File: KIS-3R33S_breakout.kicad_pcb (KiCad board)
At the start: 2 copper layers, 5 parts, among them P1 Screw terminal, P2 Screw terminal, U1 KIS-3R33S_modif

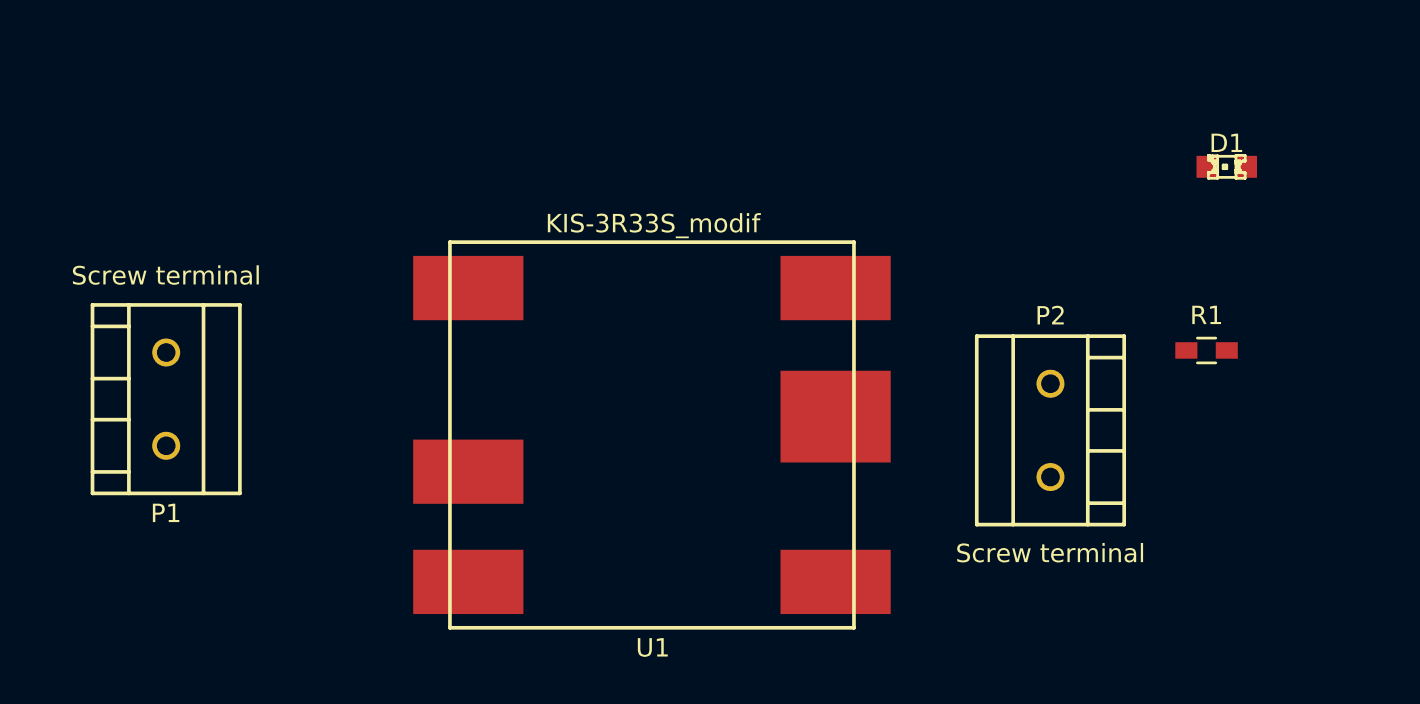
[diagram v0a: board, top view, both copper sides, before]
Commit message: Throwing parts around.
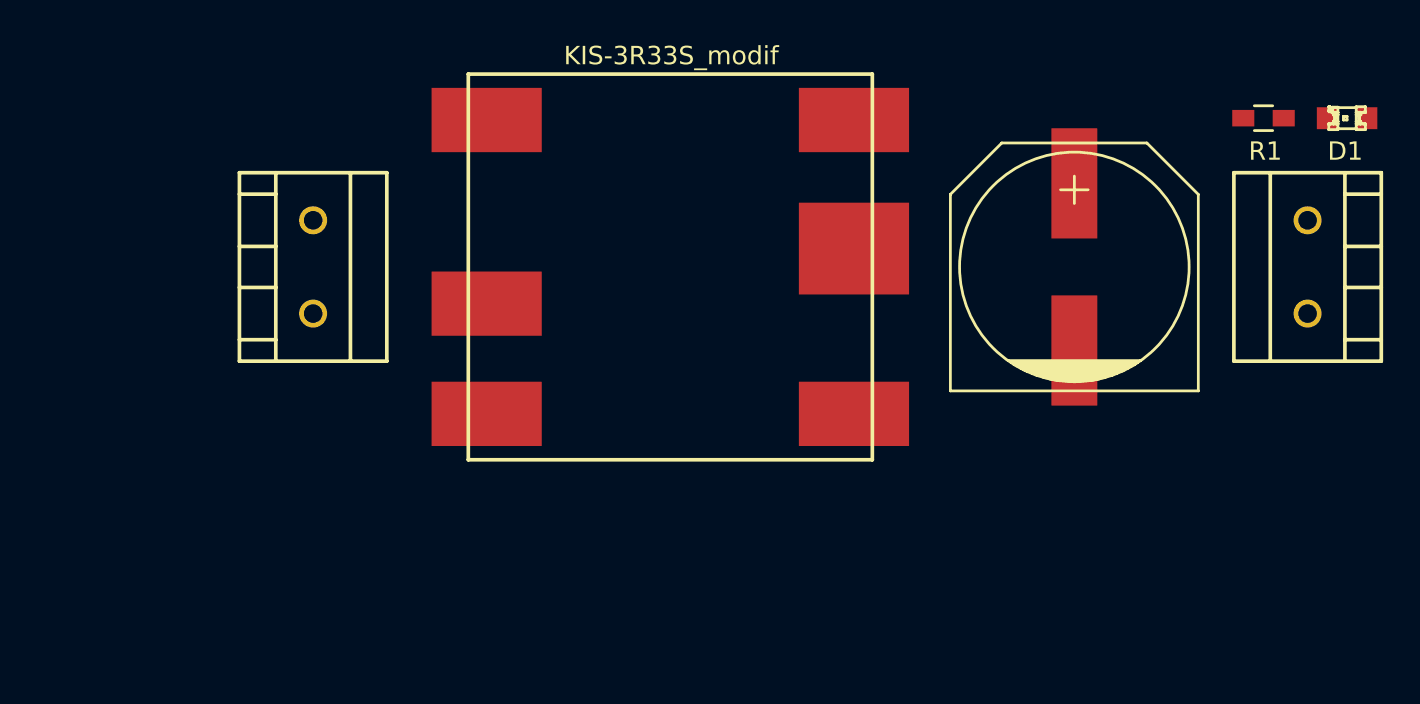
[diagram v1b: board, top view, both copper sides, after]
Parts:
- added C1: 1mF, 25V, Capacitors_SMD:c_elec_SMD_12.5x13.5, F.Cu at (172.0, 100.0)
- moved P2 16.6 mm to (184.7, 100.0)
- moved R1 13.0 mm to (182.3, 91.9)
- moved P1 10.8 mm to (130.6, 100.0)
- moved U1 9.20 mm to (150.0, 100.0)
- moved D1 7.07 mm to (186.8, 91.9)
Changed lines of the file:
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@@
 (kicad_pcb (version 4) (host pcbnew "(2015-05-01 BZR 5636)-product")
   (general
-    (links 8)
-    (no_connects 8)
-    (area 116.607142 92.155 182.14846 121.75)
+    (links 10)
+    (no_connects 10)
+    (area 124.607142 87.3 190.642858 112.6)
     (thickness 1.6)
     (drawings 0)
     (tracks 0)
     (zones 0)
-    (modules 5)
+    (modules 6)
     (nets 5)
   )
@@
   )
   (module DC-DC-modules:KIS-3R33S (layer F.Cu)
-    (at 149 109.15)
+    (at 150 100)
     (descr ./Docs/KIS-3R33S.pdf)
     (tags "DC-DC, buck, KIS-3R33S")
-    (fp_text reference U1 (at 0.05 11.6) (layer F.SilkS)
+    (fp_text reference U1 (at 0.05 11.6) (layer F.SilkS) hide
       (effects (font (size 1 1) (thickness 0.2)))
     )
@@
   )
   (module LEDs:LED-0805 (layer F.Cu)
-    (at 180.3 94.55)
+    (at 186.85 91.9)
     (descr "LED 0805 smd package")
     (tags "LED 0805 SMD")
     (attr smd)
-    (fp_text reference D1 (at 0 -1.27) (layer F.SilkS)
+    (fp_text reference D1 (at -0.1 1.8) (layer F.SilkS)
       (effects (font (size 1 1) (thickness 0.15)))
     )
@@
   )
   (module my_parts:MADW__SCREW_TERMINAL_2pin (layer F.Cu)
-    (at 122.55 107.2 180)
-    (fp_text reference P1 (at 0.01 -6.23 180) (layer F.SilkS)
-      (effects (font (size 1 1) (thickness 0.2)))
-    )
-    (fp_text value "Screw terminal" (at 0 6.71 180) (layer F.SilkS)
+    (at 130.55 100 180)
+    (fp_text reference P1 (at 0.01 -6.23 180) (layer F.SilkS) hide
+      (effects (font (size 1 1) (thickness 0.2)))
+    )
+    (fp_text value "Screw terminal" (at 0 6.71 180) (layer F.SilkS) hide
       (effects (font (size 1 1) (thickness 0.2)))
     )
@@
   )
   (module my_parts:MADW__SCREW_TERMINAL_2pin (layer F.Cu)
-    (at 170.7 108.9)
-    (fp_text reference P2 (at 0.01 -6.23) (layer F.SilkS)
-      (effects (font (size 1 1) (thickness 0.2)))
-    )
-    (fp_text value "Screw terminal" (at 0 6.71) (layer F.SilkS)
+    (at 184.7 100)
+    (fp_text reference P2 (at 0.01 -6.23) (layer F.SilkS) hide
+      (effects (font (size 1 1) (thickness 0.2)))
+    )
+    (fp_text value "Screw terminal" (at 0 6.71) (layer F.SilkS) hide
       (effects (font (size 1 1) (thickness 0.2)))
     )
@@
   )
   (module Resistors_SMD:R_0603_HandSoldering (layer F.Cu)
-    (at 179.2 104.55)
+    (at 182.3 91.9)
     (descr "Resistor SMD 0603, hand soldering")
     (tags "resistor 0603")
     (attr smd)
-    (fp_text reference R1 (at 0 -1.9) (layer F.SilkS)
+    (fp_text reference R1 (at 0.1 1.8) (layer F.SilkS)
       (effects (font (size 1 1) (thickness 0.15)))
     )
@@
     )
   )
+  (module Capacitors_SMD:c_elec_SMD_12.5x13.5 (layer F.Cu)
+    (at 172 100 90)
+    (descr "SMT capacitor, aluminium electrolytic, 12.5x13.5")
+    (fp_text reference C1 (at 8.6 -0.05 180) (layer F.SilkS) hide
+      (effects (font (size 1 1) (thickness 0.15)))
+    )
+    (fp_text value "1mF, 25V" (at 0 8 90) (layer F.Fab) hide
+      (effects (font (size 1 1) (thickness 0.15)))
+    )
+    (fp_line (start 3.95 -6.75) (end 6.75 -3.95) (layer F.SilkS) (width 0.15))
+    (fp_line (start 6.75 3.95) (end 3.95 6.75) (layer F.SilkS) (width 0.15))
+    (fp_line (start -6.15 1.1) (end -6.15 -1.1) (layer F.SilkS) (width 0.15))
+    (fp_line (start -6.1 1.35) (end -6.1 -1.35) (layer F.SilkS) (width 0.15))
+    (fp_line (start -6 -1.7) (end -6 1.7) (layer F.SilkS) (width 0.15))
+    (fp_line (start -5.9 2.05) (end -5.9 -2.05) (layer F.SilkS) (width 0.15))
+    (fp_line (start -5.8 -2.3) (end -5.8 2.3) (layer F.SilkS) (width 0.15))
+    (fp_line (start -5.7 2.55) (end -5.7 -2.55) (layer F.SilkS) (width 0.15))
+    (fp_line (start -5.6 2.75) (end -5.6 -2.75) (layer F.SilkS) (width 0.15))
+    (fp_line (start -5.5 -2.95) (end -5.5 2.95) (layer F.SilkS) (width 0.15))
+    (fp_line (start -5.4 3.1) (end -5.4 -3.1) (layer F.SilkS) (width 0.15))
+    (fp_line (start -5.3 -3.3) (end -5.3 3.3) (layer F.SilkS) (width 0.15))
+    (fp_line (start -5.2 -3.45) (end -5.2 3.45) (layer F.SilkS) (width 0.15))
+    (fp_line (start -5.1 -3.6) (end -5.1 3.6) (layer F.SilkS) (width 0.15))
+    (fp_line (start -2.2 -0.45) (end -6.9 -0.45) (layer Dwgs.User) (width 0.15))
+    (fp_line (start -2.2 0.45) (end -2.2 -0.45) (layer Dwgs.User) (width 0.15))
+    (fp_line (start -6.9 0.45) (end -2.2 0.45) (layer Dwgs.User) (width 0.15))
+    (fp_line (start -6.9 -0.45) (end -6.9 0.45) (layer Dwgs.User) (width 0.15))
+    (fp_line (start 2.2 0.45) (end 2.2 -0.45) (layer Dwgs.User) (width 0.15))
+    (fp_line (start 6.9 0.45) (end 2.2 0.45) (layer Dwgs.User) (width 0.15))
+    (fp_line (start 6.9 -0.45) (end 6.9 0.45) (layer Dwgs.User) (width 0.15))
+    (fp_line (start 2.2 -0.45) (end 6.9 -0.45) (layer Dwgs.User) (width 0.15))
+    (fp_line (start -6.75 6.75) (end -6.75 -6.75) (layer F.SilkS) (width 0.15))
+    (fp_line (start 3.95 6.75) (end -6.75 6.75) (layer F.SilkS) (width 0.15))
+    (fp_line (start 6.75 -3.95) (end 6.75 3.95) (layer F.SilkS) (width 0.15))
+    (fp_line (start -6.75 -6.75) (end 3.95 -6.75) (layer F.SilkS) (width 0.15))
+    (fp_circle (center 0 0) (end 6.25 0) (layer F.SilkS) (width 0.15))
+    (fp_line (start 4.95 0) (end 3.45 0) (layer F.SilkS) (width 0.15))
+    (fp_line (start 4.2 -0.75) (end 4.2 0.75) (layer F.SilkS) (width 0.15))
+    (pad 1 smd rect (at 4.55 0 90) (size 6 2.5) (layers F.Cu F.Paste F.Mask)
+      (net 1 /Vout))
+    (pad 2 smd rect (at -4.55 0 90) (size 6 2.5) (layers F.Cu F.Paste F.Mask)
+      (net 4 GND))
+  )
 )

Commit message: Done?
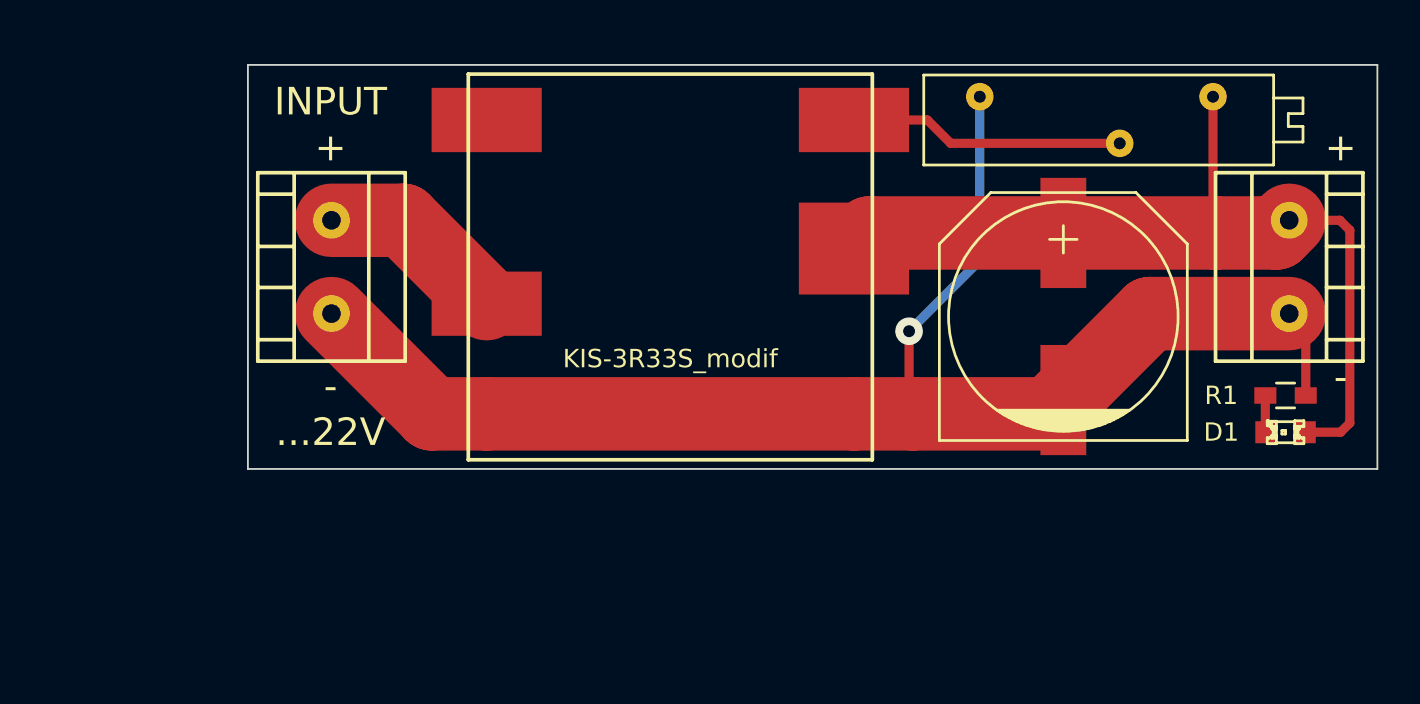
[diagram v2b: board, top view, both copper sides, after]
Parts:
- added G***: LED_smile_silkscreen_6mm, led-smile:LED_smile_silkscreen_6mm, B.Cu at (160.0, 100.0)
- added G***: OSHW-logo_silkscreen_6mm, oshw-logo:OSHW-logo_silkscreen_6mm, B.Cu at (140.0, 100.0)
- added RV1: 100k, Potentiometers:trimmer-pot_side-adjust_TSR-3006P_TH, F.Cu at (173.2, 92.0)
- moved D1 17.4 mm to (183.5, 109.0)
- moved R1 15.1 mm to (183.5, 107.0)
- moved C1 2.77 mm to (171.4, 102.7)
- moved P1 1.00 mm to (131.6, 100.0)
- moved P2 1.00 mm to (183.7, 100.0)
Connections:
- U1 pad 6: (no net) -> /ADJ
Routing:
- net GND: track 0.00 -> 80.5 mm, vias 0 -> 1
- net /Vout: track 0.00 -> 48.5 mm
- net /ADJ: track 0.00 -> 15.0 mm
- net /Vin: track 0.00 -> 10.3 mm
- net Net-(D1-Pad1): track 0.00 -> 2.02 mm
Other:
- board outline added: 61.5 x 22 mm
- net class Default: trace_width 0.25 -> 0.5; via_dia 0.6 -> 1.5; via_drill 0.4 -> 0.65
- net class power added: clearance 0.2, trace_width 4, via_dia 1.5, via_drill 0.65
- board text added: "+"
- board text added: "-"
- board text added: "...22V"
- board text added: "INPUT"
- board text added: "KIS-3R33S_breakout 2015 - blog.spitzenpfeil.org"
